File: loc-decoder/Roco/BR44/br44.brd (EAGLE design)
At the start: 17 x 38 mm, 8 parts

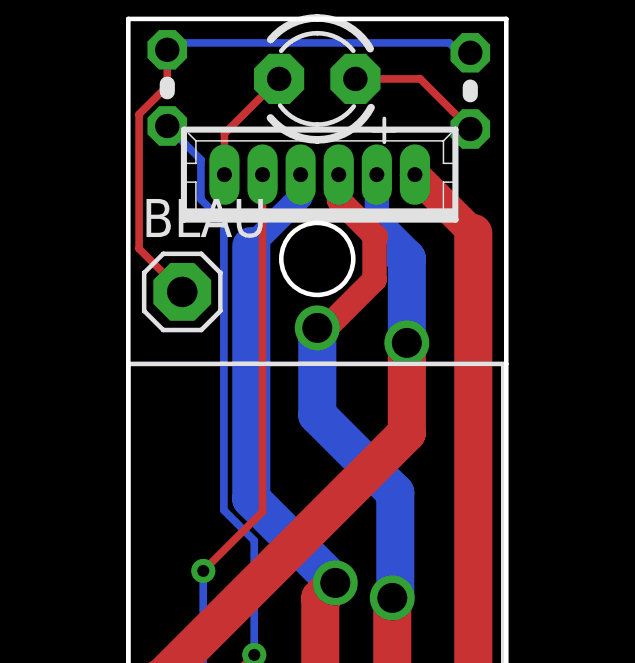
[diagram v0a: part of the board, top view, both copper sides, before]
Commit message: misc
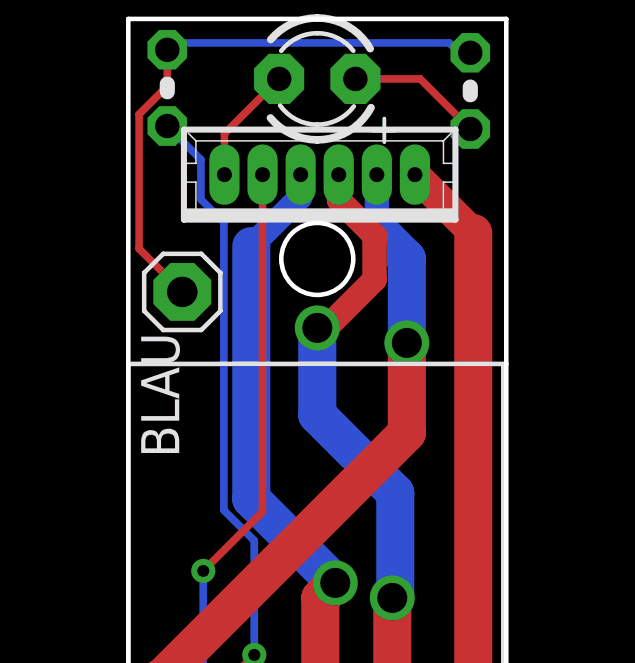
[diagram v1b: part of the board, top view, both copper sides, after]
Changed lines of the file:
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@@
 <?xml version="1.0" encoding="utf-8"?>
 <!DOCTYPE eagle SYSTEM "eagle.dtd">
-<eagle version="9.4.0">
+<eagle version="9.5.2">
 <drawing>
 <settings>
@@
 </element>
 <element name="BLAU" library="adafruit" library_urn="urn:adsk.eagle:library:420" package="1X01" package3d_urn="urn:adsk.eagle:package:6240654/1" value="" x="4" y="28.9" smashed="yes">
-<attribute name="NAME" x="2.6538" y="30.7288" size="1.27" layer="25" ratio="10"/>
+<attribute name="NAME" x="2.6288" y="27.5462" size="1.27" layer="25" ratio="10" rot="R270"/>
 <attribute name="VALUE" x="2.73" y="25.725" size="1.27" layer="27"/>
 </element>

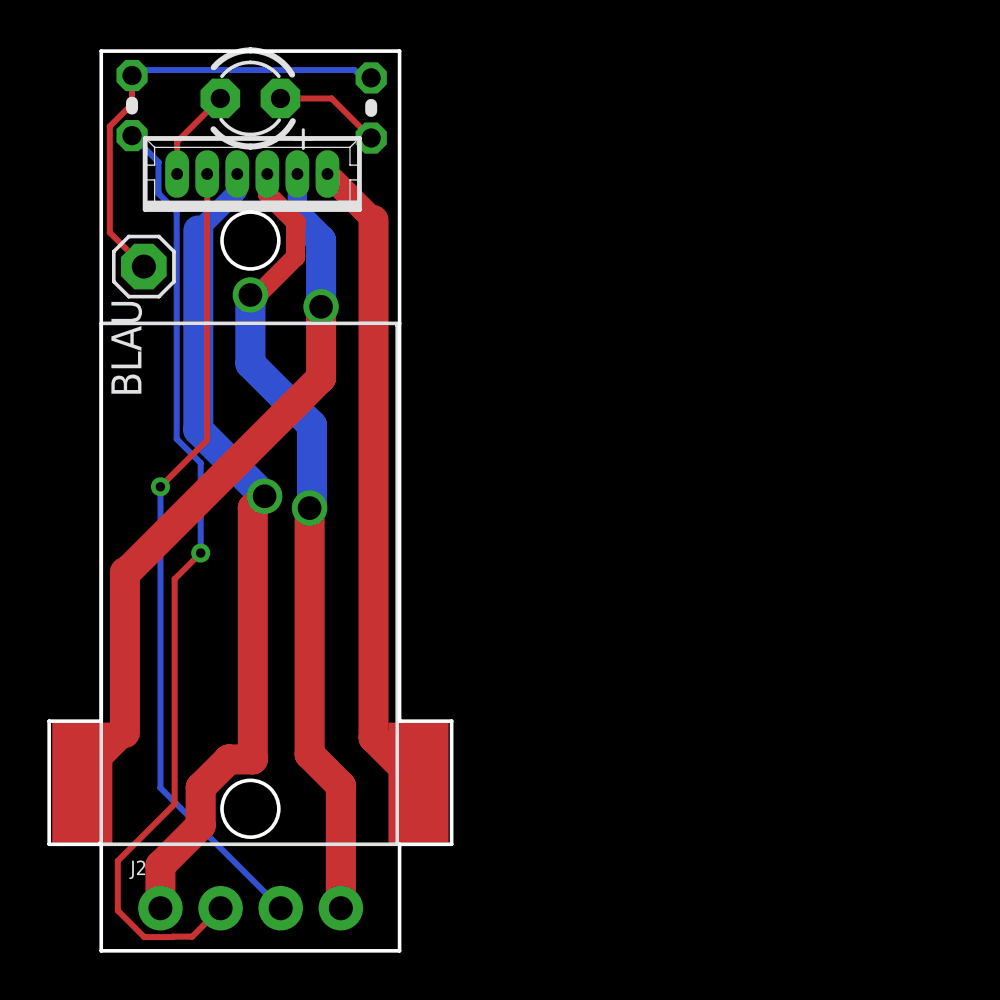
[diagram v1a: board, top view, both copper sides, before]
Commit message: misc
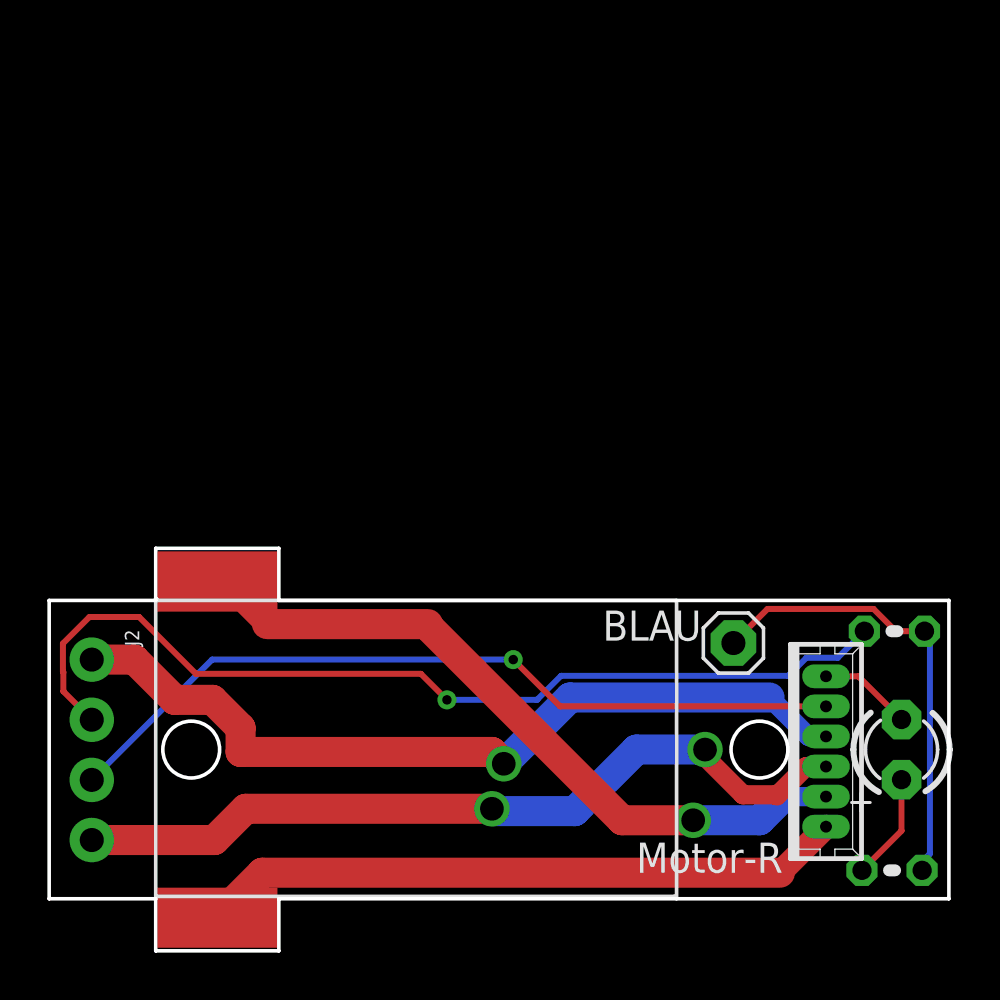
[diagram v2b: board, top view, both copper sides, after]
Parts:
- moved R3 39.1 mm to (35.7, 13.5), turned to 0 degrees
- moved R4 39.0 mm to (35.6, 3.40), turned to 0 degrees
- moved LED2 38.9 mm to (36.0, 8.50), turned to 90 degrees
- moved U$1 34.4 mm to (32.8, 8.42), turned to 270 degrees
- moved BLAU 29.5 mm to (28.9, 13.0), turned to 270 degrees
- moved J2 10.9 mm to (1.80, 12.3), turned to 270 degrees
- moved PAD1 10.2 mm to (7.10, 1.40), turned to 270 degrees
- moved PAD2 10.2 mm to (7.10, 15.6), turned to 270 degrees
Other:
- board size 17 x 38 mm -> 38 x 17 mm
- board text added: "Motor-R"
- board text added: "https://github.com/stb49078/nscale-adapter-decoder"
